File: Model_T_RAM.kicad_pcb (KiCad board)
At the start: 2 copper layers, 19.8 x 34.3 mm, 4 parts, among them J1 KC-85_RAM, U1 6264, U2 74HC86

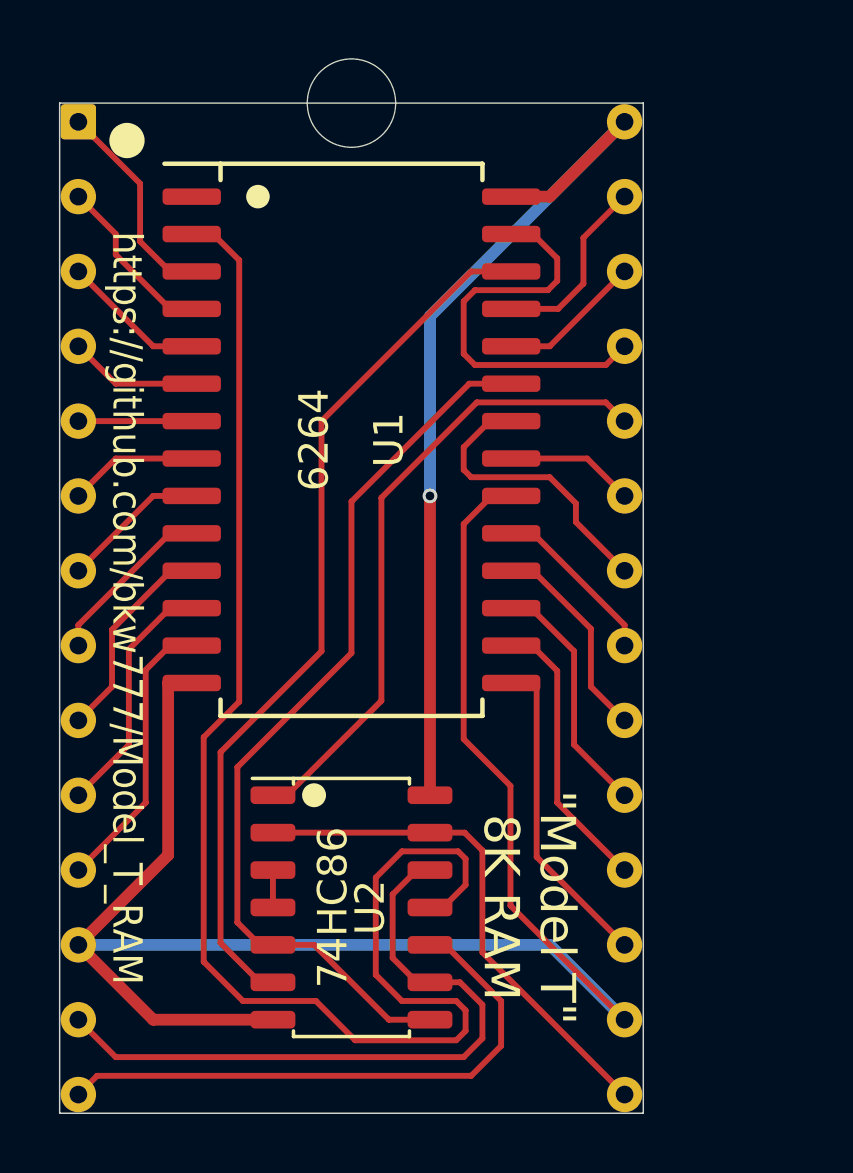
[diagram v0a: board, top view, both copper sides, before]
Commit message: rotate 7486
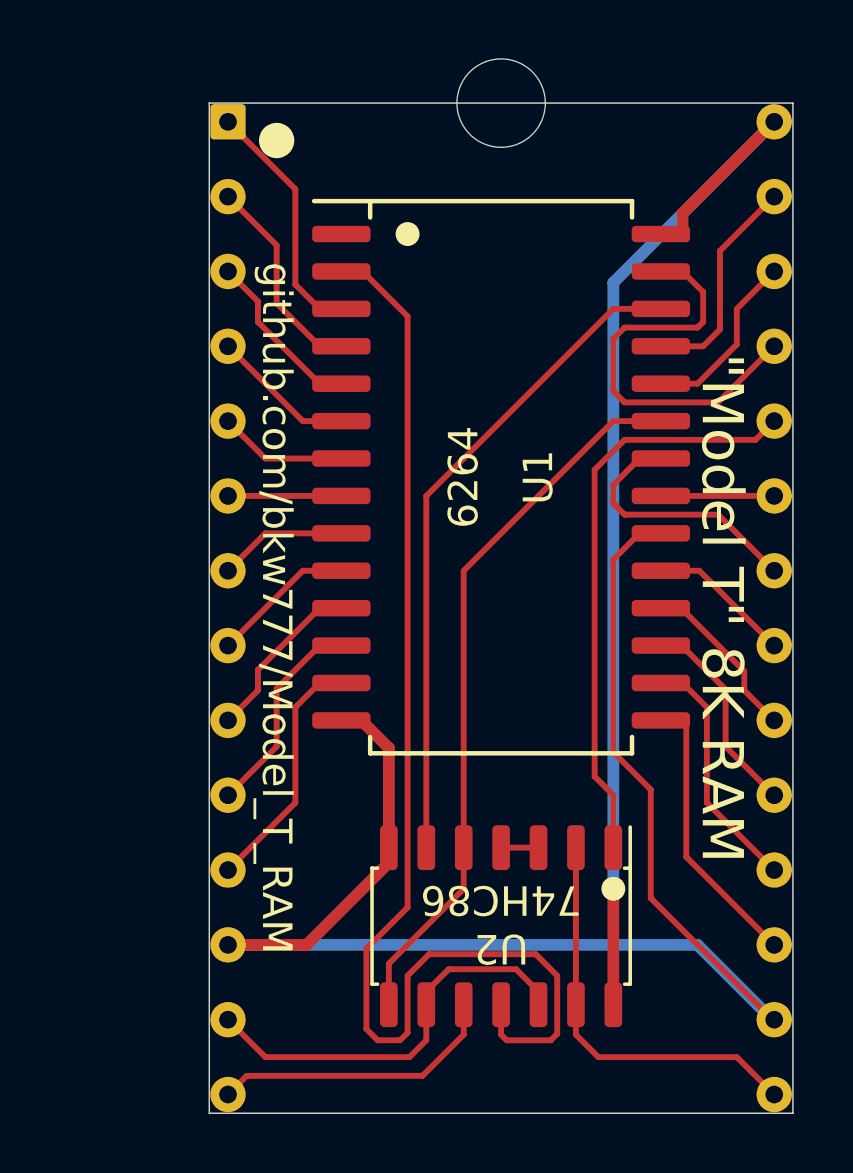
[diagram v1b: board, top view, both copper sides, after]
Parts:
- U2: footprint 000_LOCAL:SOIC-14_3.9x8.7mm_P1.27mm -> 000_LOCAL:SOIC-14_4x9
- moved U1 5.24 mm to (147.3, 94.6)
- moved U2 5.12 mm to (147.3, 109.9), turned to 270 degrees
- moved J1 5.08 mm to (147.3, 99.1)
- moved REF** 5.08 mm to (147.3, 81.9)
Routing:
- net /~CS_B: track 19.8 -> 9.86 mm
- net /~CS_A: track 23.1 -> 14.0 mm
- net /A12: track 49.9 -> 42.0 mm
- net /CE2: track 30.0 -> 22.5 mm
- net GND: track 59.3 -> 52.1 mm
- net VCC: track 30.5 -> 37.3 mm
- net /A11: track 30.9 -> 24.6 mm
- net /~CS_C: track 17.6 -> 13.9 mm
- net /~CS_D: track 21.8 -> 19.9 mm
- net /AD6: track 7.11 -> 5.81 mm
- net /AD2: track 9.65 -> 8.38 mm
- net /AD1: track 8.38 -> 7.11 mm
- net /AD3: track 11.0 -> 9.72 mm
- net /A7: track 7.11 -> 8.38 mm
- net /A6: track 5.84 -> 7.11 mm
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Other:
- board text added: ""Model T" 8K RAM"
- board text added: "github.com/bkw777/Model_T_RAM"
- board text added: "v004 alt"
- board text removed: ""Model T""
- board text removed: "8K RAM"
- board text removed: "https://github.com/bkw777/Model_T_RAM"
- board text removed: "v004"
